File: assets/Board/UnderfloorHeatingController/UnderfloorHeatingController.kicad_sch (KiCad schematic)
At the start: 10 parts, among them J2 Screw_Terminal_01x03, J3 Screw_Terminal_01x03, U2 Waveshare_ESP32-S3-Tiny

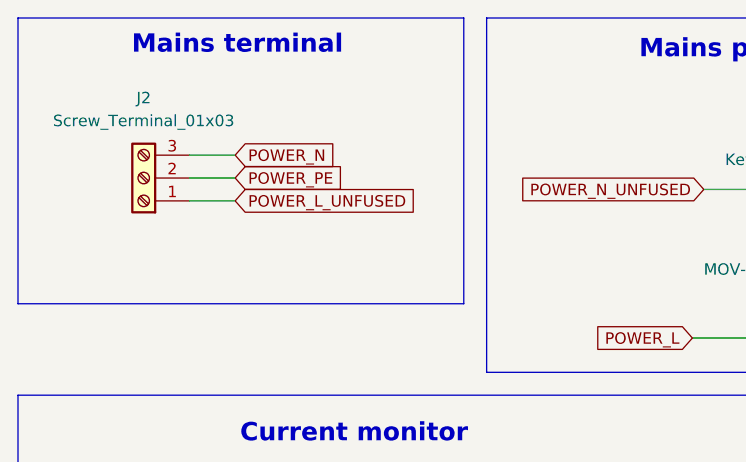
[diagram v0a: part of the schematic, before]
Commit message: Layout fixes.
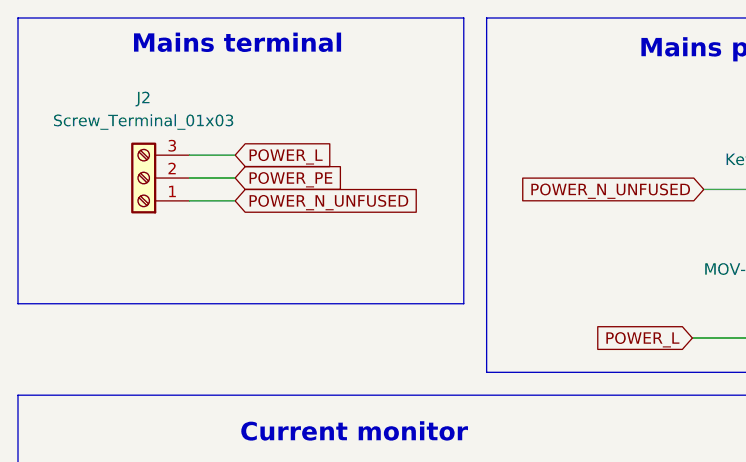
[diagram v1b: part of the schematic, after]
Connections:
- net POWER_L_UNFUSED is gone; now on net POWER_N_UNFUSED: J2.1 (Pin_1)
- net POWER_L: now also J2.3 (Pin_3)
- net POWER_N: no longer J2.3 (Pin_3)
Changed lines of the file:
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@@
 		)
 	)
-	(global_label "POWER_N"
+	(global_label "POWER_L"
 		(shape input)
 		(at 38.1 29.21 0)
@@
 		)
 		(property "Intersheetrefs" "${INTERSHEET_REFS}"
-			(at 49.8542 29.21 0)
+			(at 49.5518 29.21 0)
 			(effects
 				(font
@@
 		)
 	)
-	(global_label "POWER_L_UNFUSED"
+	(global_label "POWER_N_UNFUSED"
 		(shape input)
 		(at 38.1 34.29 0)
@@
 		)
 		(property "Intersheetrefs" "${INTERSHEET_REFS}"
-			(at 59.228 34.29 0)
+			(at 59.5304 34.29 0)
 			(effects
 				(font
